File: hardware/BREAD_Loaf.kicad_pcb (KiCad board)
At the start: 2 copper layers, 35.4 x 50.7 mm, 29 parts, among them J1 PPPC101LGBN-RC, J2 THING_PLUS_LOGICAL, Q1 BSS138, Q2 BSS138, Q3 BSS138, U1 AP63205WU-7, U2 LTC4311ISC6-TRMPBF

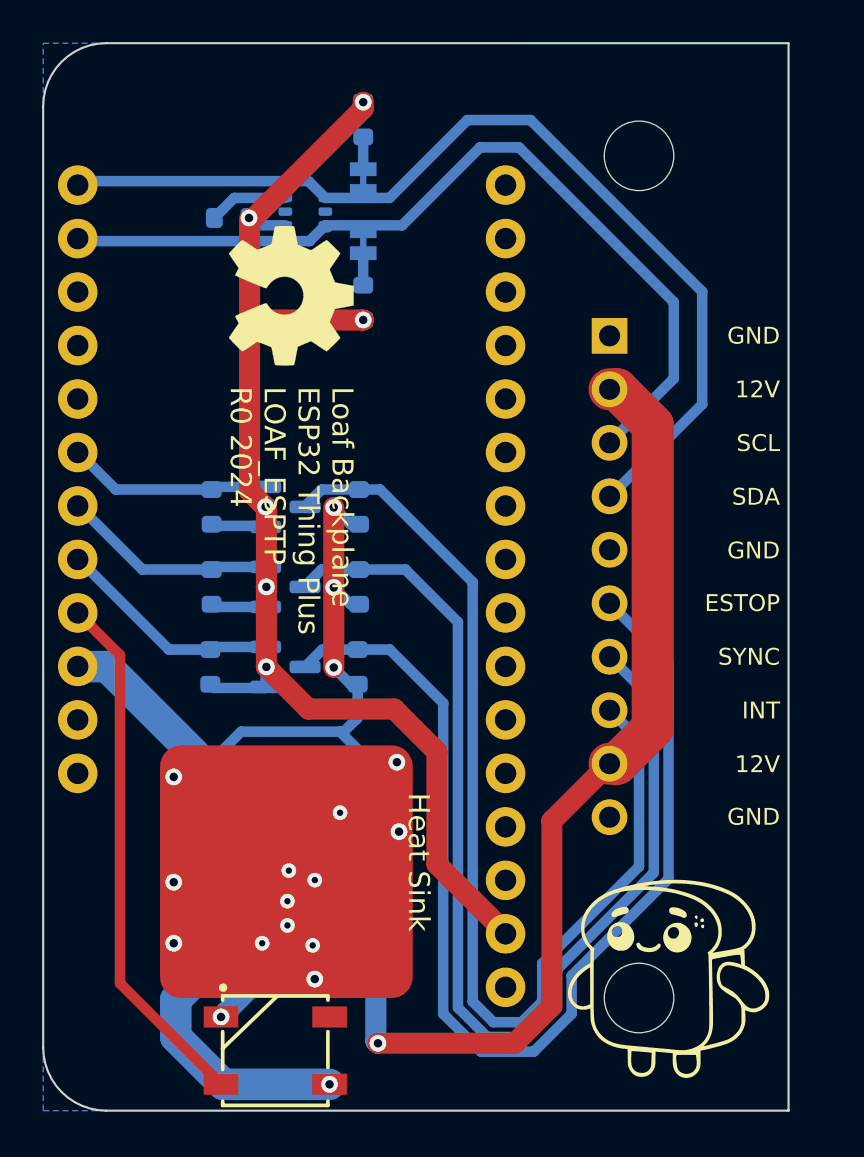
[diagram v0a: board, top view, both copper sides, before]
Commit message: JLCPCB order rev-A
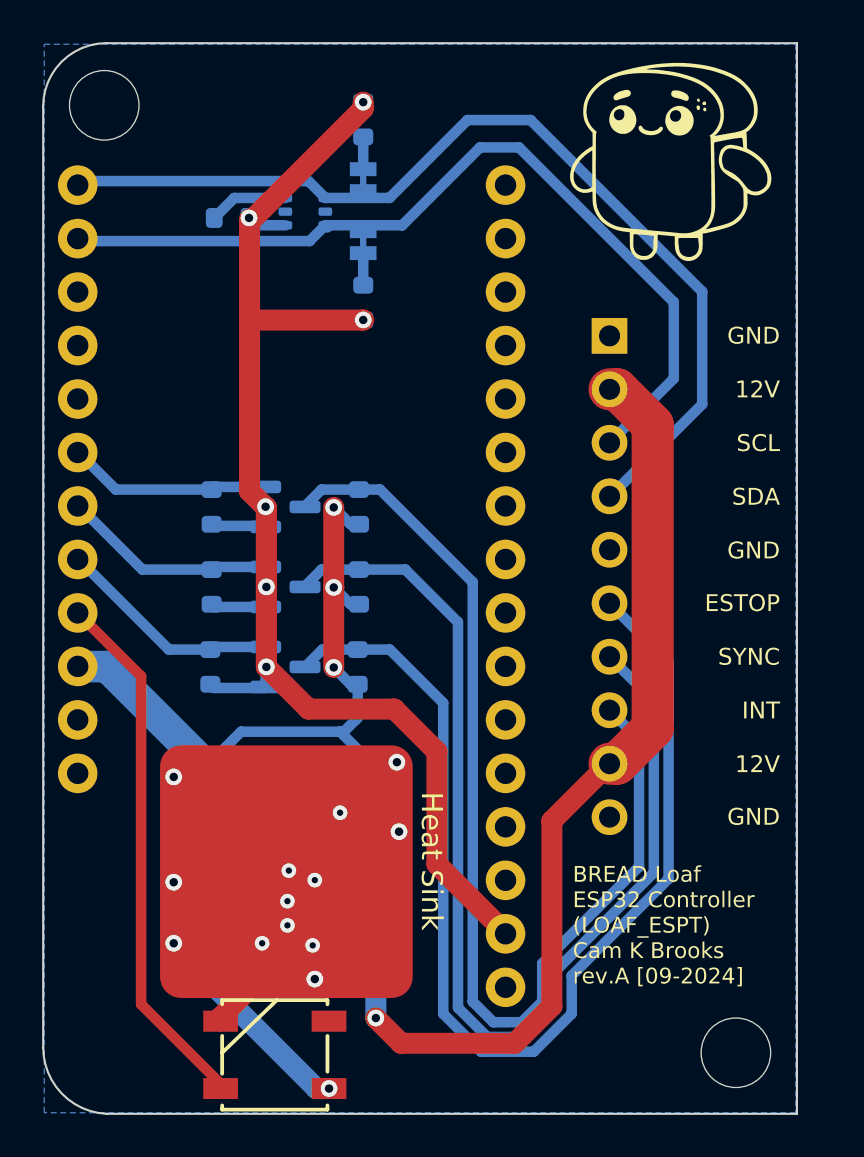
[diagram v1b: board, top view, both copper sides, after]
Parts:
- removed Logo1: Logo_Open_Hardware_Small, Symbol:OSHW-Symbol_6.7x6mm_SilkScreen
- added REF**: OSHW-Logo2_9.8x8mm_SilkScreen, Symbol:OSHW-Logo2_9.8x8mm_SilkScreen, B.Cu at (82.5, 78.3)
- moved demo** 38.8 mm to (77.7, 83.6)
- moved ST1 25.5 mm to (55.9, 76.0)
- moved ST2 5.28 mm to (85.9, 121.0)
- moved D1 0.20 mm to (64.0, 121.0)
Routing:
- net +5V: track 60.0 -> 56.6 mm
- net +12V: track 51.3 -> 50.6 mm
- net GND: track 2.89 -> 3.08 mm, vias 14 -> 13
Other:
- board size 35.4 x 50.7 mm -> 35.8 x 50.9 mm
- board text added: "BREAD Loaf ESP32 Controller (LOAF_ESPT) Cam K Brooks rev.A [09-2024]"
- board text removed: "Loaf Backplane ESP32 Thing Plus LOAF_ESPTP R0 2024"
